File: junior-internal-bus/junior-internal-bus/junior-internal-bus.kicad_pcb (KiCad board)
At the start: 2 copper layers, 115.6 x 45.7 mm, 6 parts, among them J1 C64AC, J2 C64AC, J3 Conn_01x06_Male

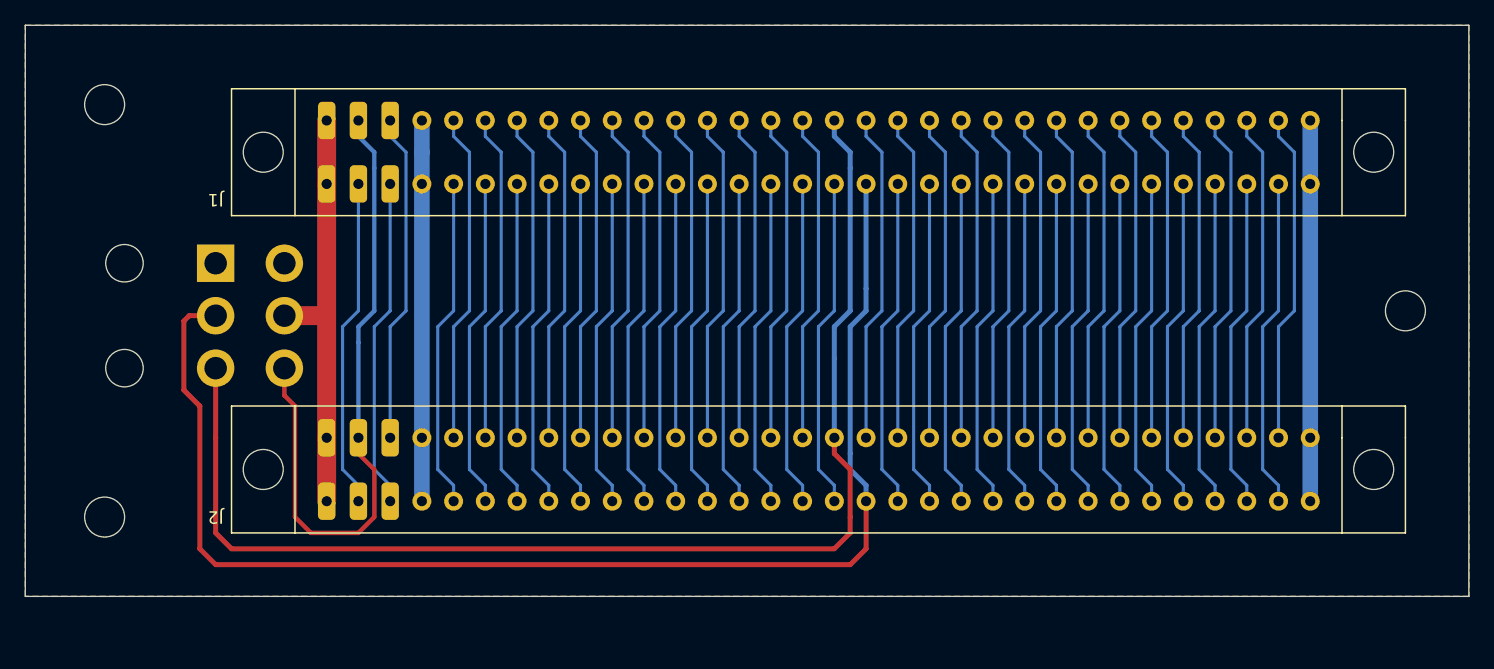
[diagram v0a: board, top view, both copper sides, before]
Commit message: junior bus
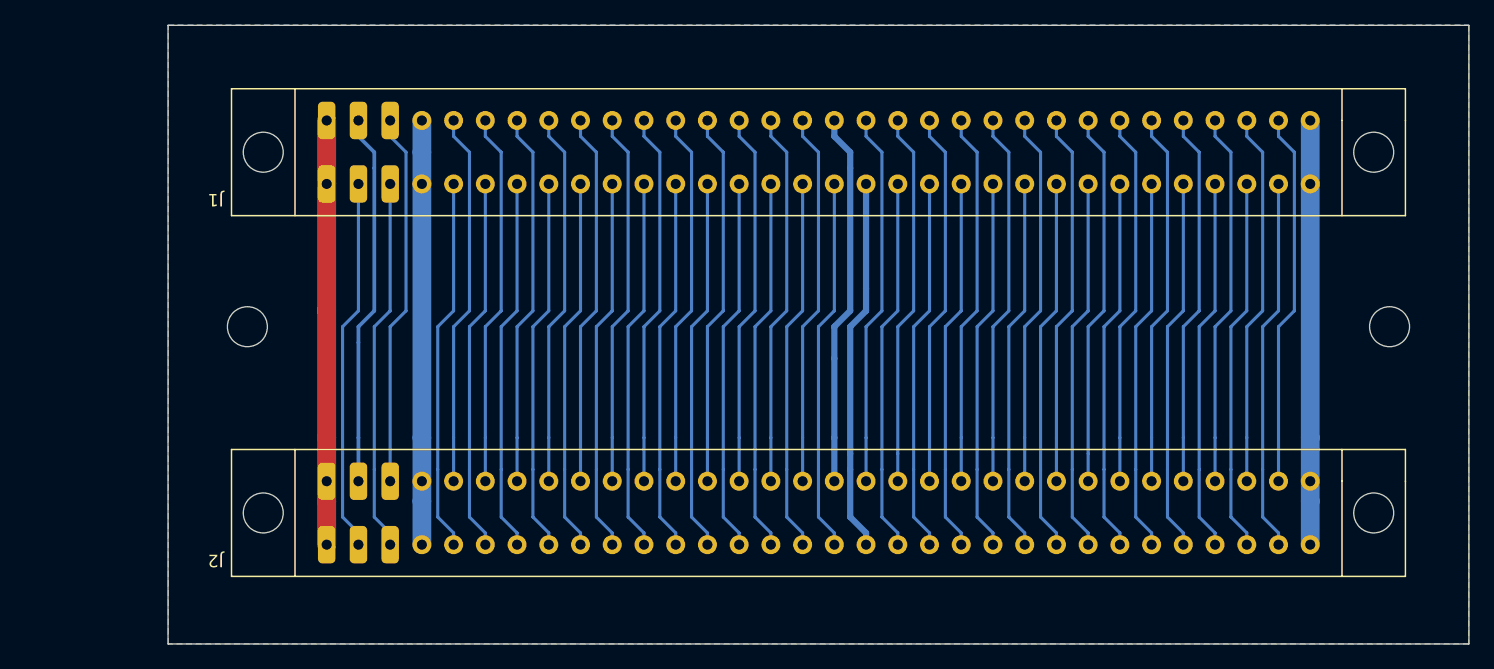
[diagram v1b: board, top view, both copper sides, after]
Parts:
- removed J3: Conn_01x06_Male, Connectors_Molex:Molex_MiniFit-JR-5569-06A2_2x03x4.20mm_Angled
- removed the REF** at (73.7, 64.8)
- moved REF** 19.1 mm to (85.1, 82.5)
- moved J2 3.48 mm to (91.4, 100.0)
- moved REF** 1.80 mm to (176.5, 82.5)
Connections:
- net +12V renamed Net-(J1-PadC17)
- net +5V renamed Net-(J1-PadA1)
- net -12V renamed Net-(J1-PadC2)
- net -5V renamed Net-(J1-PadA18)
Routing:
- net Net-(J1-PadA18): track 107.0 -> 29.9 mm
- net Net-(J1-PadC17): track 99.7 -> 29.9 mm
- net Net-(J1-PadC2): track 53.0 -> 29.8 mm
- net GND: track 61.0 -> 67.9 mm
- net Net-(J1-PadA8): track 26.5 -> 29.9 mm
- net Net-(J1-PadA6): track 26.5 -> 29.9 mm
- net Net-(J1-PadA5): track 26.5 -> 29.9 mm
- net Net-(J1-PadA15): track 26.5 -> 29.9 mm
- net Net-(J1-PadA14): track 26.5 -> 29.9 mm
- net Net-(J1-PadA13): track 26.5 -> 29.9 mm
- net Net-(J1-PadA12): track 26.5 -> 29.9 mm
- net Net-(J1-PadA10): track 26.5 -> 29.9 mm
- net Net-(J1-PadC9): track 26.5 -> 29.9 mm
- net Net-(J1-PadC8): track 26.5 -> 29.9 mm
- net Net-(J1-PadC7): track 26.5 -> 29.9 mm
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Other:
- board size 115.6 x 45.7 mm -> 104.1 x 49.5 mm
